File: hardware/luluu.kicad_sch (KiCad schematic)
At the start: 50 parts, among them CN1 DISP_LCD_ST7789, J1 BATT_CON, J2 SWD_PI_3WIRE, J3 STEMMA_{QT} I_{2}C (JST SH), J4 Micro_SD_Card, J5 UART_PI_3WIRE, J6 USB_C_Receptacle_USB2.0, Q1 DMG3415UFY4Q-7, Q2 BSS138, SW1 SW_USBBOOT, SW2 SW_RESET, U1 W25Q128JVSS, U2 RT9080-33GJ5, U3 RP2040, U4 MCP73831-2-OT, U5 APX803, Y1 TX322512M4LBCE2T

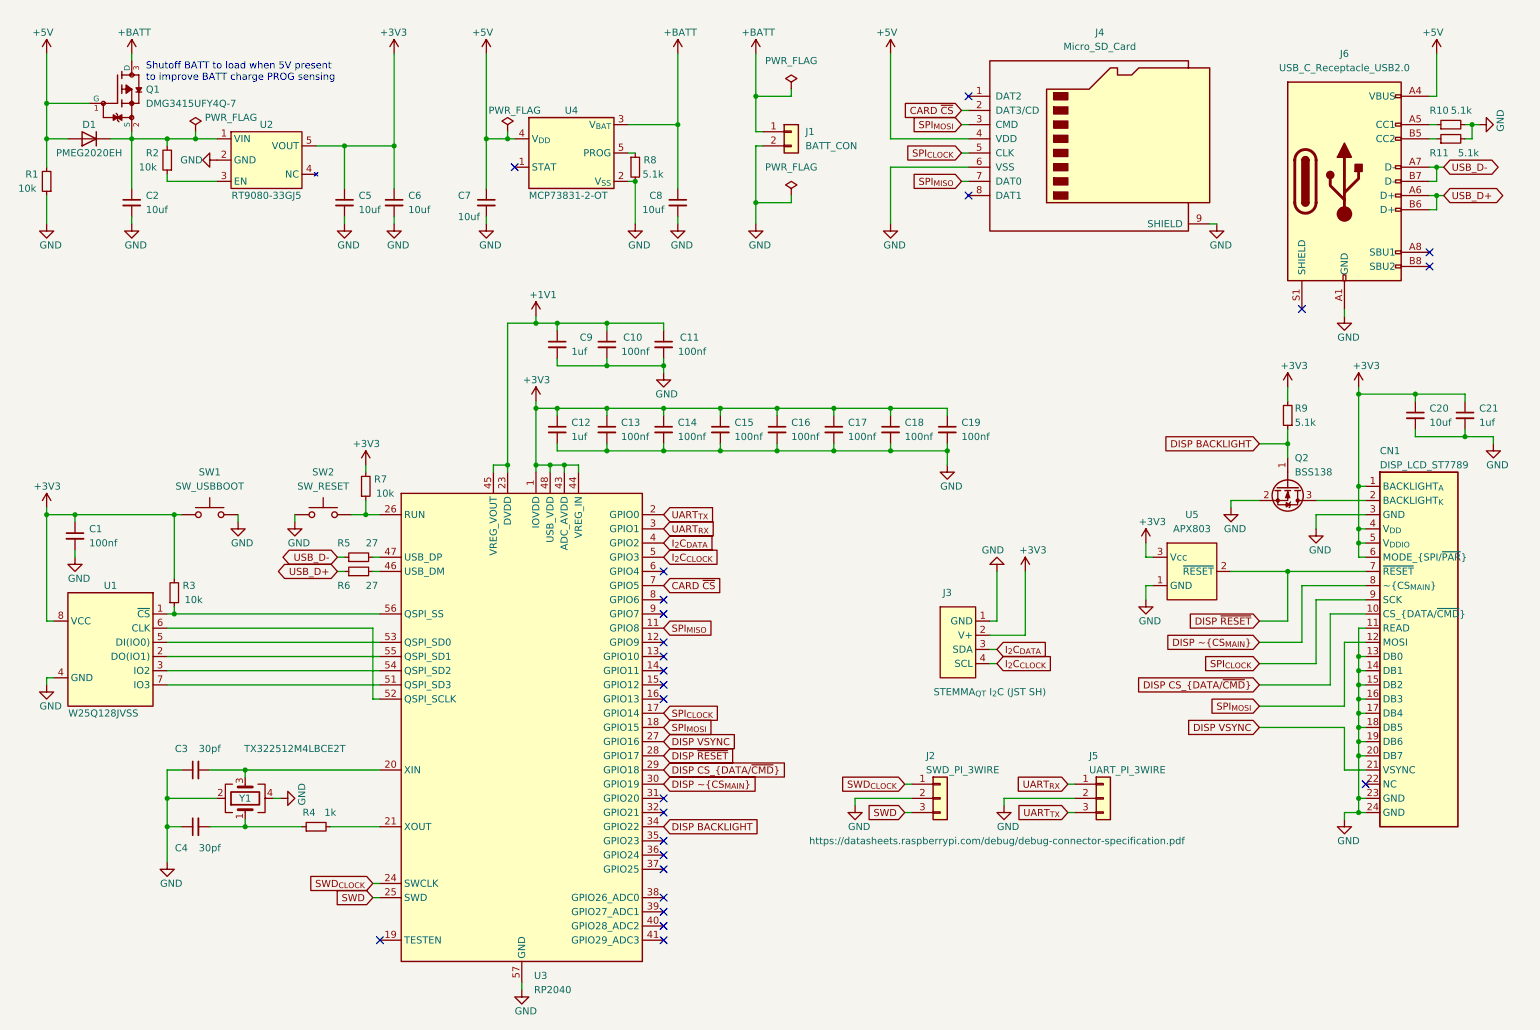
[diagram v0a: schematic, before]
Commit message: lots of updates
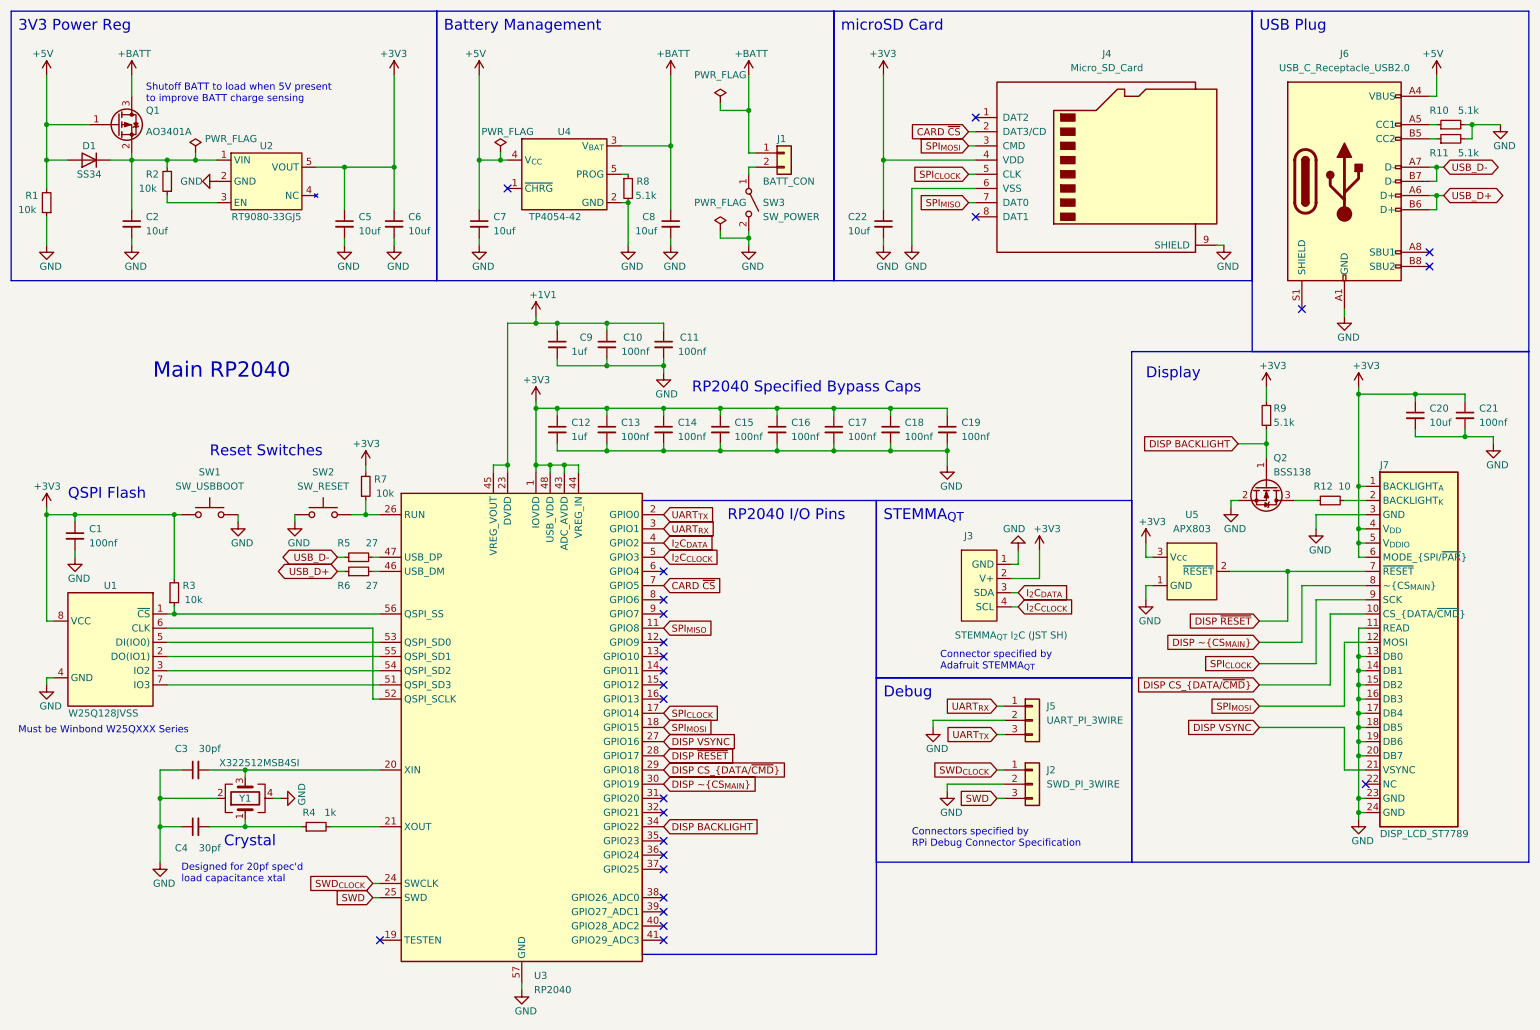
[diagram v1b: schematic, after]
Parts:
- added C22: 10uf, Capacitor_SMD:C_0603_1608Metric_Pad1.08x0.95mm_HandSolder, symbol Device:C_Small
- added R12: 10, Resistor_SMD:R_0603_1608Metric_Pad0.98x0.95mm_HandSolder, symbol Device:R_Small
- added SW3: SW_POWER, Button_Switch_SMD:SW_SPDT_PCM12, symbol Switch:SW_SPST
- C1, C10, C11, C13, C14, C15, C16, C17, C18, C19: LCSC (none) -> C1525
- C12, C9: LCSC (none) -> C15849
- C2, C20, C5, C6, C7, C8: LCSC (none) -> C96446
- C21: value 1uf -> 100nf; footprint Capacitor_SMD:C_0603_1608Metric_Pad1.08x0.95mm_HandSolder -> Capacitor_SMD:C_0402_1005Metric_Pad0.74x0.62mm_HandSolder; LCSC (none) -> C1525
- C3, C4: LCSC (none) -> C1570
- D1: value PMEG2020EH -> SS34; footprint (none) -> Diode_SMD:D_SMA_Handsoldering; LCSC (none) -> C8678
- J4: LCSC (none) -> C585350
- J6: LCSC (none) -> C2988369
- J7: renamed from CN1; footprint (none) -> luluu:FPC_24_JUSHUO_AFC04-S24XCA-00; Connector Datasheet (none) -> https://datasheet.lcsc.com/lcsc/2010201934_JUSHUO-AFC04-S24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; LCSC (none) -> C883644
- Q1: value DMG3415UFY4Q-7 -> AO3401A; footprint luluu:TRANS_DMG3415UFY4Q-7 -> Package_TO_SOT_SMD:SOT-23; symbol luluu:DMG3415UFY4Q-7 -> Transistor_FET:AO3401A; LCSC (none) -> C15127
- Q2: LCSC (none) -> C7420339
- R1, R2, R3, R7: footprint (none) -> Resistor_SMD:R_0603_1608Metric_Pad0.98x0.95mm_HandSolder; LCSC (none) -> C25804
- R10, R11, R8, R9: footprint (none) -> Resistor_SMD:R_0603_1608Metric_Pad0.98x0.95mm_HandSolder; LCSC (none) -> C23186
- R4: footprint (none) -> Resistor_SMD:R_0603_1608Metric_Pad0.98x0.95mm_HandSolder; LCSC (none) -> C21190
- R5, R6: footprint (none) -> Resistor_SMD:R_0603_1608Metric_Pad0.98x0.95mm_HandSolder; LCSC (none) -> C25190
- SW1, SW2: footprint luluu:TS-1187A-B-A-B -> Button_Switch_SMD:SW_Push_1P1T_XKB_TS-1187A; LCSC (none) -> C318884
- U1: LCSC (none) -> C97521
- U2: LCSC (none) -> C841192
- U3: LCSC (none) -> C2040
- U4: value MCP73831-2-OT -> TP4054-42; symbol luluu:MCP73831-2-OT -> luluu:TP4054-42; LCSC (none) -> C32574
- U5: LCSC (none) -> C526393
- Y1: value TX322512M4LBCE2T -> X322512MSB4SI; LCSC (none) -> C9002
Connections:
- net +3V3: now also J4.4 (VDD), C22.1
- net +5V: no longer J4.4 (VDD)
- net GND: now also C22.2, SW3.2 (B); no longer J1.2 (Pin_2)
- net at Q2.3 (D): now also R12.1; no longer J7.2 (BACKLIGHT_{K})
- new net: J1.2 (Pin_2), SW3.1 (A)
- new net: J7.2 (BACKLIGHT_{K}), R12.2
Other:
- note added: "3V3 Power Reg"
- note added: "Battery Management"
- note added: "Connector specified by Adafruit STEMMA_{QT}"
- note added: "Connectors specified by RPi Debug Connector Specification"
- note added: "Crystal"
- note added: "Debug"
- note added: "Designed for 20pf spec'd load capacitance xtal"
- note added: "Display"
- note added: "Main RP2040"
- note added: "Must be Winbond W25QXXX Series"
- note added: "QSPI Flash"
- note added: "RP2040 I/O Pins"
- note added: "RP2040 Specified Bypass Caps"
- note added: "Reset Switches"
- note added: "STEMMA_{QT}"
- note added: "Shutoff BATT to load when 5V present to improve BATT charge sensing"
- note added: "USB Plug"
- note added: "microSD Card"
- note removed: "Shutoff BATT to load when 5V present to improve BATT charge PROG sensing"
- moved on the sheet: C2, C5, C6, C7, C8, D1, J1, J2, J3, J4, J5, Q2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
